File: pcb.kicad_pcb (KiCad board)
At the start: 2 copper layers, 76 parts, among them SW1 SW_Push, U1 ATmega32U4-AU, Y1 16MHz

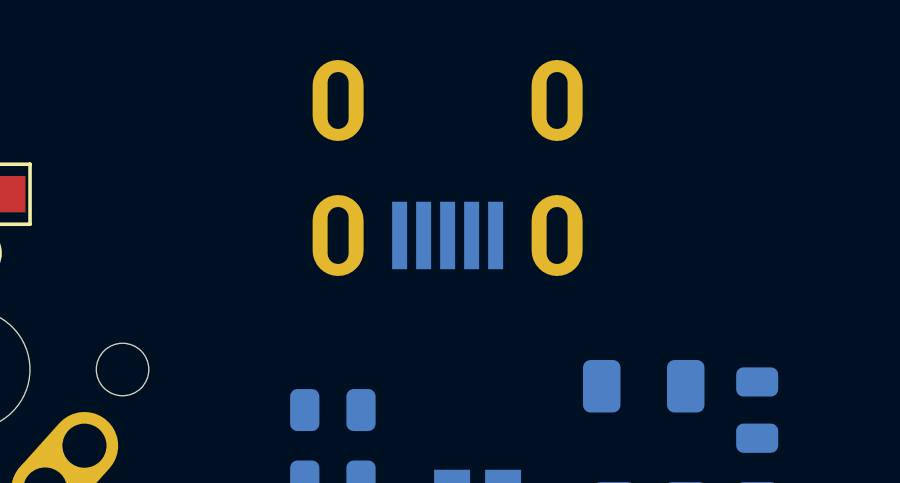
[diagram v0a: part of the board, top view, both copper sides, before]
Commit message: Attempt 1
Attempt 1
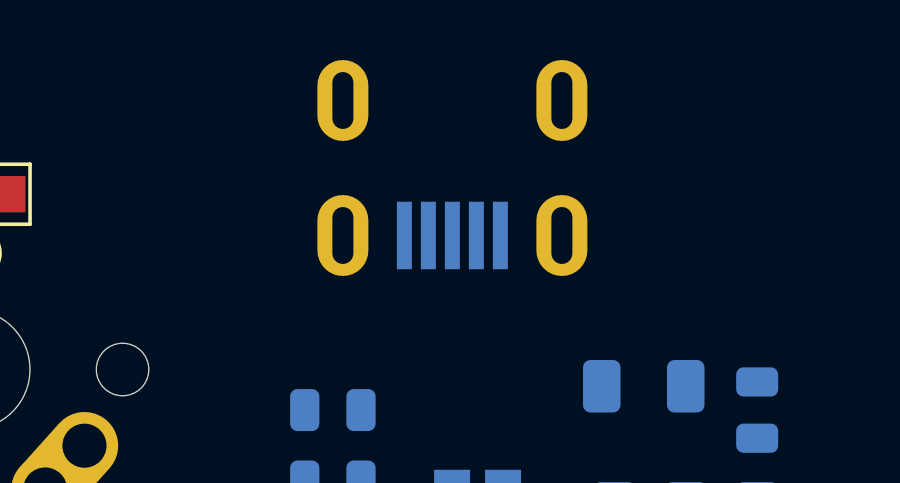
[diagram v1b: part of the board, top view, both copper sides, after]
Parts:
- moved USB1 0.16 mm to (142.2, 91.3)
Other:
- net class Default removed
